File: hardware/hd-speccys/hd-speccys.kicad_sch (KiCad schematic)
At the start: 13 parts, among them J1 PI_ZERO_2x20, J2 ULA_ZX_02x20, J3 ULA_SOCKET_02x20, U1 74LS541, U2 74LS132, U3 74LS541

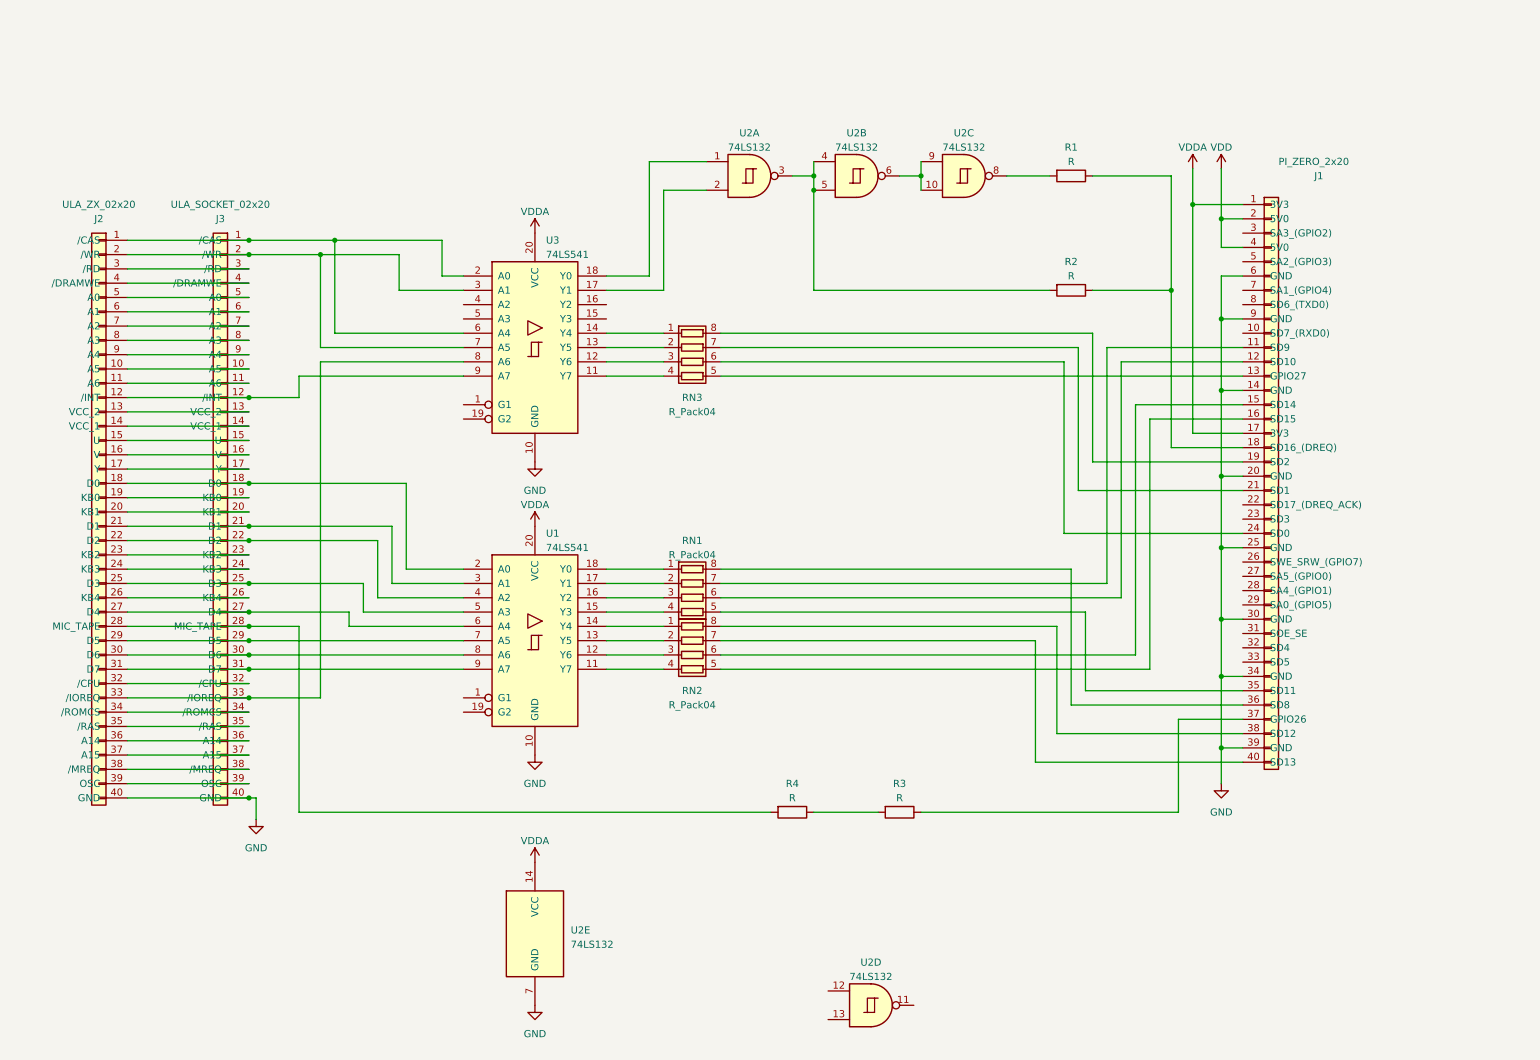
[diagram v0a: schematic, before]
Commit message: wip: PCB prototype/schematic
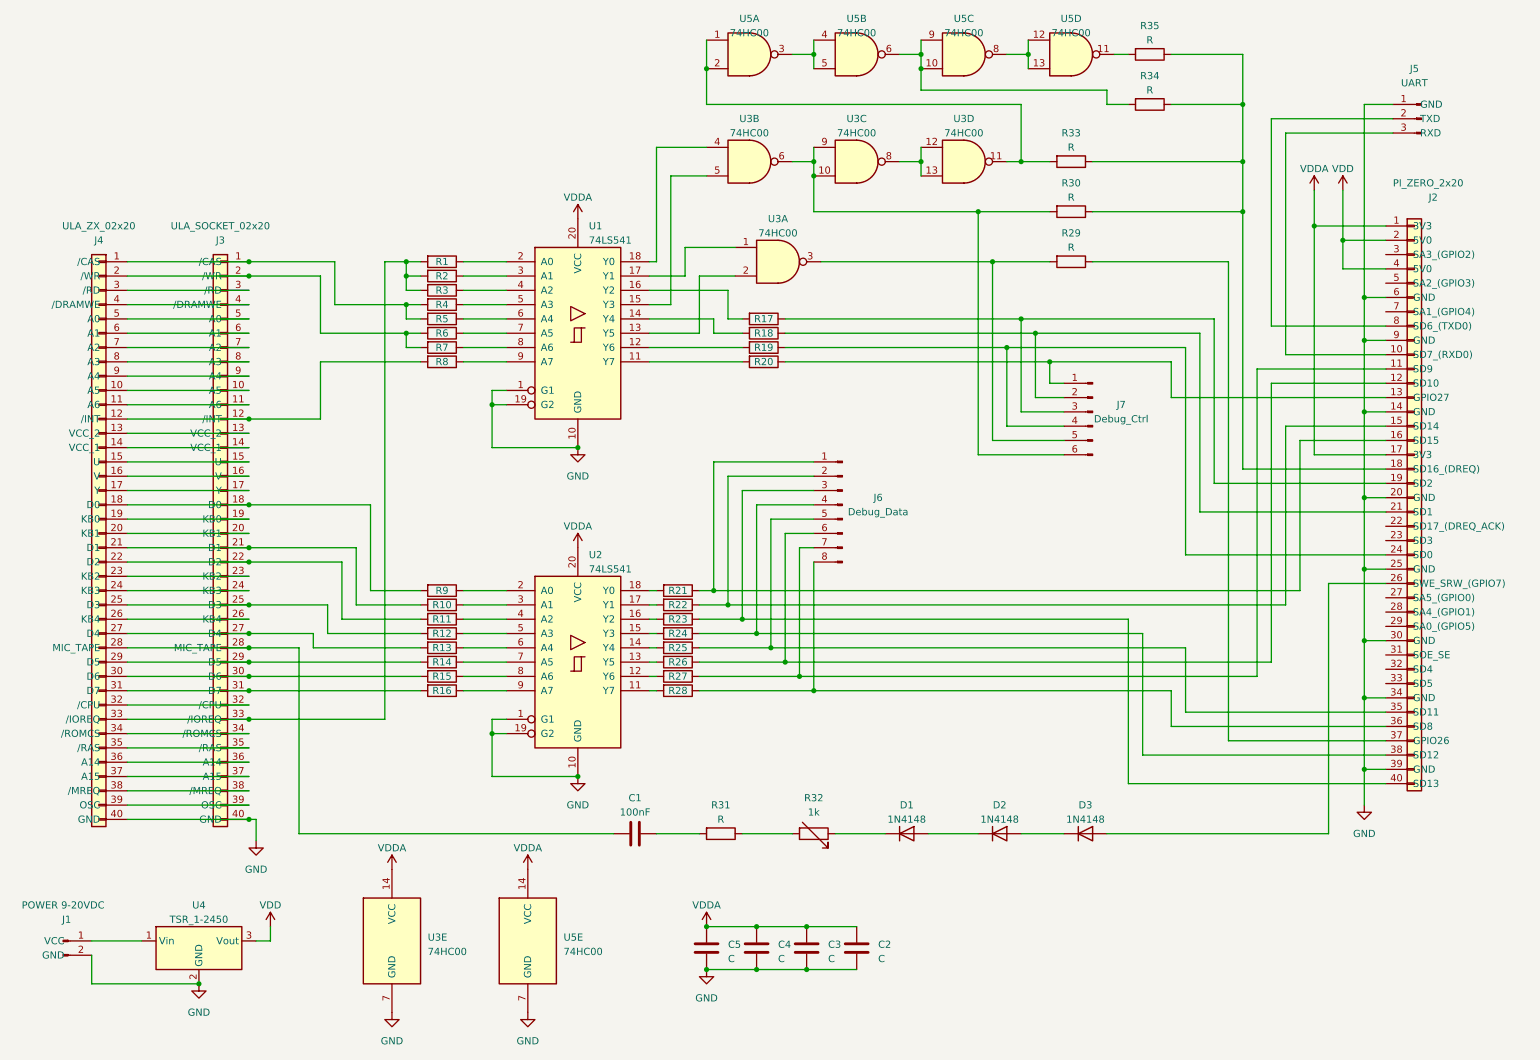
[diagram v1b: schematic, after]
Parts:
- removed RN1, RN2, RN3: R_Pack04, symbol Device:R_Pack04
- removed U2: 74LS132, symbol 74xx:74LS132
- added C1: 100nF, Capacitor_SMD:C_0603_1608Metric_Pad1.08x0.95mm_HandSolder, symbol Device:C
- added C2, C3, C4, C5: C, Capacitor_SMD:C_0603_1608Metric_Pad1.08x0.95mm_HandSolder, symbol Device:C
- added D1, D2, D3: 1N4148, Diode_SMD:D_SOD-323_HandSoldering, symbol Diode:1N4148
- added J1: POWER 9-20VDC, Connector_PinHeader_2.54mm:PinHeader_1x02_P2.54mm_Horizontal, symbol Connector:Conn_01x02_Pin
- added J5: UART, Connector_PinHeader_2.54mm:PinHeader_1x03_P2.54mm_Vertical, symbol Connector:Conn_01x03_Pin
- added J6: Debug_Data, Connector_PinHeader_2.54mm:PinHeader_1x08_P2.54mm_Vertical, symbol Connector:Conn_01x08_Pin
- added J7: Debug_Ctrl, Connector_PinHeader_2.54mm:PinHeader_1x06_P2.54mm_Vertical, symbol Connector:Conn_01x06_Pin
- added R1, R10, R11, R12, R13, R14, R15, R16, R17, R18, R19, R2, R20, R21, R22, R23, R24, R25, R26, R27, R28, R3, R31, R34, R35, R5, R6, R7, R8, R9: R, Resistor_SMD:R_0603_1608Metric_Pad0.98x0.95mm_HandSolder, symbol Device:R
- added R32: 1k, Potentiometer_SMD:Potentiometer_Bourns_TC33X_Vertical, symbol Device:R_Variable
- added U3, U5: 74HC00, Package_SO:TSSOP-14_4.4x5mm_P0.65mm, symbol 74xx:74HC00
- added U4: TSR_1-2450, Converter_DCDC:Converter_DCDC_TRACO_TSR-1_THT, symbol Regulator_Switching:TSR_1-2450
- J2: renamed from J1; footprint (none) -> Module:Raspberry_Pi_Zero_Socketed_THT_FaceDown_MountingHoles
- J3: footprint (none) -> Package_DIP:DIP-40_W15.24mm_Socket
- J4: renamed from J2; footprint (none) -> Package_DIP:DIP-40_W15.24mm_Socket
- R29: renamed from R3; footprint (none) -> Resistor_SMD:R_0603_1608Metric_Pad0.98x0.95mm_HandSolder
- R30: renamed from R2; footprint (none) -> Resistor_SMD:R_0603_1608Metric_Pad0.98x0.95mm_HandSolder
- R33: renamed from R1; footprint (none) -> Resistor_SMD:R_0603_1608Metric_Pad0.98x0.95mm_HandSolder
- R4: footprint (none) -> Resistor_SMD:R_0603_1608Metric_Pad0.98x0.95mm_HandSolder
- U1: renamed from U3; footprint (none) -> Package_SO:TSSOP-20_4.4x6.5mm_P0.65mm
- U2: renamed from U1; footprint (none) -> Package_SO:TSSOP-20_4.4x6.5mm_P0.65mm
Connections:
- net GND: now also U1.1 (G1), U1.19 (G2), U2.1 (G1), U2.19 (G2), C2.2, C3.2, C4.2, C5.2, J1.2 (GND), J5.1 (GND), U3.7 (GND), U4.2 (GND), U5.7 (GND)
- net VDD: now also U4.3 (Vout)
- net VDDA: now also C2.1, C3.1, C4.1, C5.1, U3.14 (VCC), U5.14 (VCC)
- net at U1.14 (Y4): now also R18.2
- net at U1.13 (Y5): now also U3.2
- net at U1.12 (Y6): now also R19.2
- net at U1.11 (Y7): now also R20.2
- net at J2.13 (GPIO27): now also J7.1 (Pin_1), R20.1
- net at J2.24 (SD0): now also J7.4 (Pin_4), R19.1
- net at J2.21 (SD1): now also J7.2 (Pin_2), R18.1
- net at J2.19 (SD2): now also J7.3 (Pin_3), R17.1
- net at R29.2: now also J7.5 (Pin_5), U3.3; no longer R4.1
- net at J3.28 (MIC_TAPE), J4.28 (MIC_TAPE): now also C1.2; no longer R4.2
- net at U1.15 (Y3): now also U3.5
- net at U1.16 (Y2): now also R17.2
- net at U1.17 (Y1): now also U3.1
- net at U1.18 (Y0): now also U3.4
- net at J3.1 (/CAS), J4.1 (/CAS): now also R4.2, R5.2; no longer U1.2 (A0), U1.6 (A4)
- net at J3.2 (/WR), J4.2 (/WR): now also R6.2, R7.2; no longer U1.3 (A1), U1.7 (A5)
- net at U1.4 (A2): now also R3.1
- net at U1.5 (A3): now also R4.1
- net at J3.33 (/IOREQ), J4.33 (/IOREQ): now also R1.2, R2.2, R3.2; no longer U1.8 (A6)
- net at J3.12 (/INT), J4.12 (/INT): now also R8.2; no longer U1.9 (A7)
- net at U2.18 (Y0): now also R21.2
- net at U2.17 (Y1): now also R22.2
- net at U2.16 (Y2): now also R23.2
- net at U2.15 (Y3): now also R24.2
- net at J2.35 (SD11): now also J6.5 (Pin_5), R25.1
- net at J2.12 (SD10): now also J6.6 (Pin_6), R26.1
- net at J2.11 (SD9): now also J6.7 (Pin_7), R27.1
- net at J2.36 (SD8): now also J6.8 (Pin_8), R28.1
- net at J3.18 (D0), J4.18 (D0): now also R9.2; no longer U2.2 (A0)
- net at J3.21 (D1), J4.21 (D1): now also R10.2; no longer U2.3 (A1)
- net at J3.22 (D2), J4.22 (D2): now also R11.2; no longer U2.4 (A2)
- net at J3.25 (D3), J4.25 (D3): now also R12.2; no longer U2.5 (A3)
- net at J3.27 (D4), J4.27 (D4): now also R13.2; no longer U2.6 (A4)
- net at J3.29 (D5), J4.29 (D5): now also R14.2; no longer U2.7 (A5)
- net at J3.30 (D6), J4.30 (D6): now also R15.2; no longer U2.8 (A6)
- net at J3.31 (D7), J4.31 (D7): now also R16.2; no longer U2.9 (A7)
- net at J2.18 (SD16_(DREQ)), R30.1, R33.1: now also R34.1, R35.1
- net at R33.2: now also U3.11, U5.1, U5.2
- net at R30.2: now also J7.6 (Pin_6), U3.10, U3.6, U3.9
- net at U2.14 (Y4): now also R25.2
- net at U2.13 (Y5): now also R26.2
- net at U2.12 (Y6): now also R27.2
- net at U2.11 (Y7): now also R28.2
- net at J2.16 (SD15): now also J6.1 (Pin_1), R21.1
- net at J2.15 (SD14): now also J6.2 (Pin_2), R22.1
- net at J2.40 (SD13): now also J6.3 (Pin_3), R23.1
- net at J2.38 (SD12): now also J6.4 (Pin_4), R24.1
- net at J2.10 (SD7_(RXD0)): now also J5.3 (RXD)
- net at J2.26 (SWE_SRW_(GPIO7)): now also D3.2 (A)
- net at J2.8 (SD6_(TXD0)): now also J5.2 (TXD)
- new net: J1.1 (VCC), U4.1 (Vin)
- new net: D2.2 (A), D3.1 (K)
- new net: R6.1, U1.7 (A5)
- new net: R34.2, U5.10, U5.6, U5.9
- new net: U5.12, U5.13, U5.8
- new net: R2.1, U1.3 (A1)
- new net: R35.2, U5.11
- new net: R5.1, U1.6 (A4)
- new net: R10.1, U2.3 (A1)
- new net: R31.1, R32.2
- new net: C1.1, R31.2
- new net: R1.1, U1.2 (A0)
- new net: R7.1, U1.8 (A6)
- new net: R8.1, U1.9 (A7)
- new net: D1.1 (K), R32.1
- new net: R15.1, U2.8 (A6)
- new net: R9.1, U2.2 (A0)
- new net: R16.1, U2.9 (A7)
- new net: U5.3, U5.4, U5.5
- new net: R11.1, U2.4 (A2)
- new net: R14.1, U2.7 (A5)
- new net: R13.1, U2.6 (A4)
- new net: D1.2 (A), D2.1 (K)
- new net: R12.1, U2.5 (A3)
- new net: U3.12, U3.13, U3.8
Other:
- moved on the sheet: J2, J3, J4, R29, R30, R33, U1, U2
